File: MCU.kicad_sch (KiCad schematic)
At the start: 13 parts, among them U1 BMD-350-A-R, Y1 32.768kHz

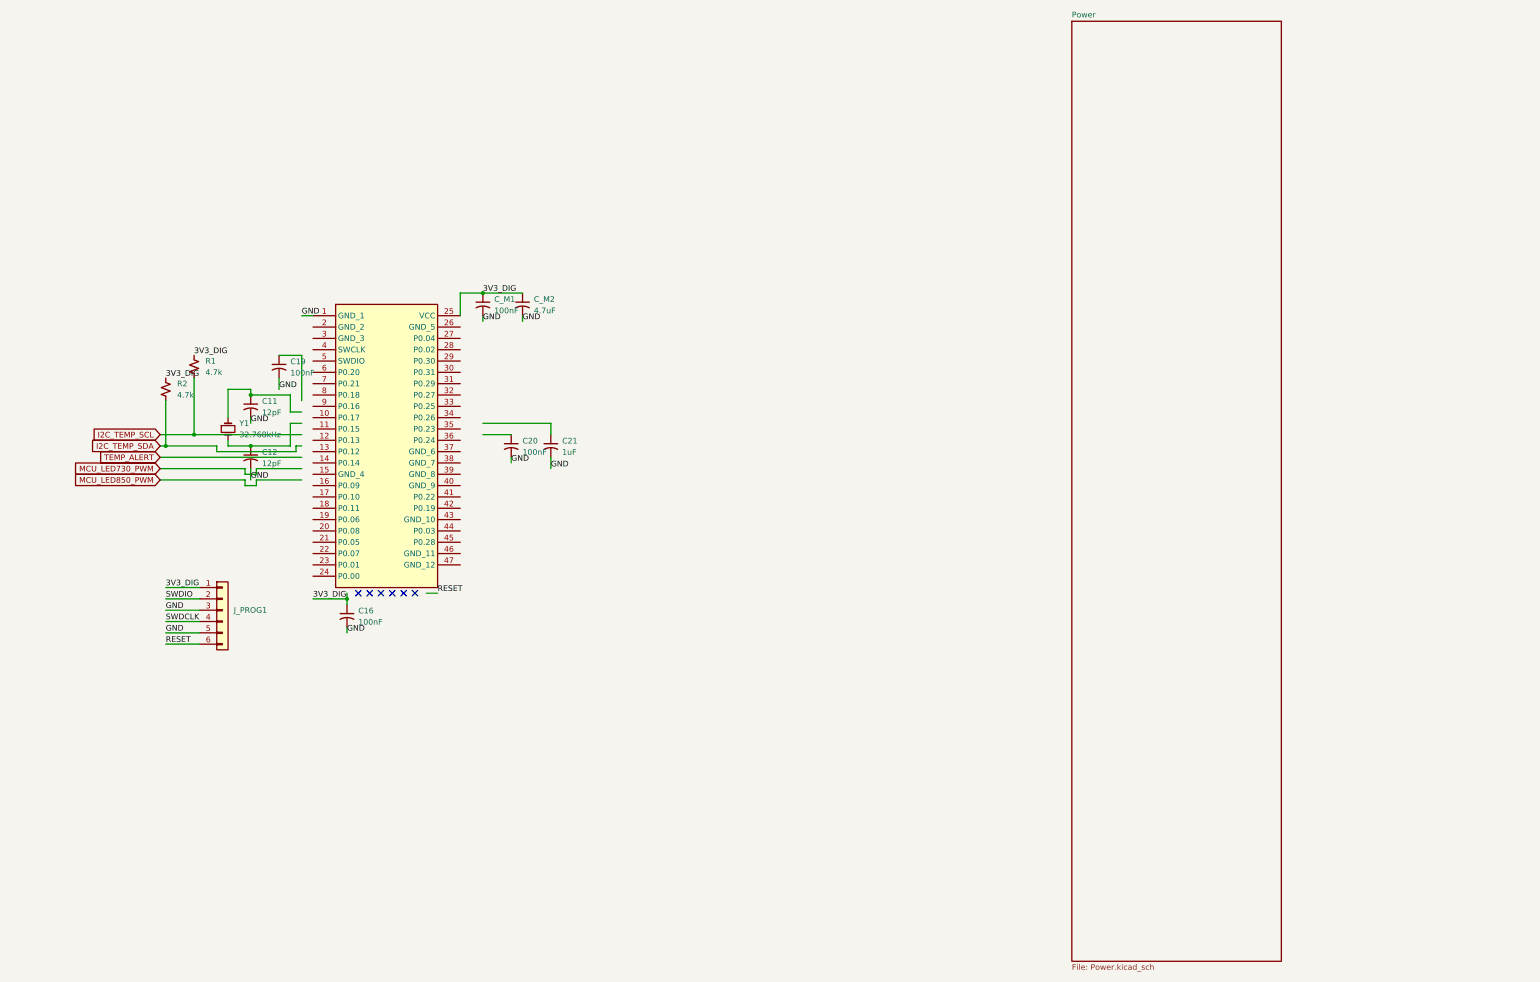
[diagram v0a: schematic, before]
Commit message: power
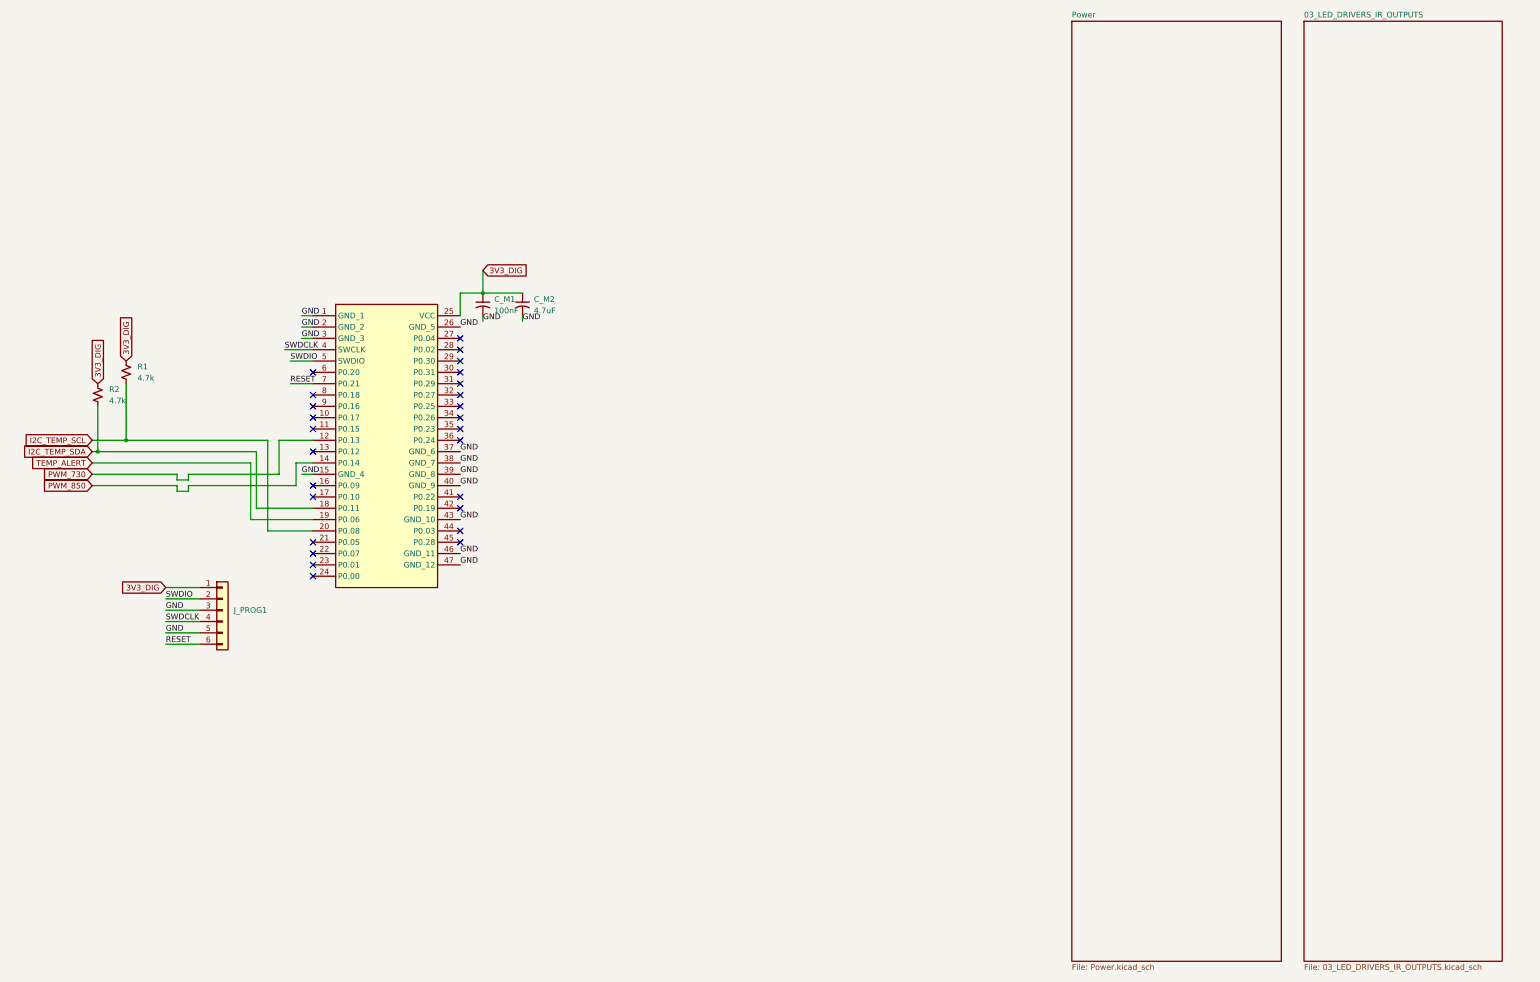
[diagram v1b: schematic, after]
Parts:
- removed C11, C12: 12pF, symbol Device:C_Small_US
- removed C16, C19, C20: 100nF, symbol Device:C_Small_US
- removed C21: 1uF, symbol Device:C_Small_US
- removed Y1: 32.768kHz, symbol Device:Crystal_Small
- U1: footprint BMD-350 -> BMD-350-A-R:BMD-350
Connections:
- net GND: now also U1.15 (GND_4), U1.2 (GND_2), U1.26 (GND_5), U1.3 (GND_3), U1.37 (GND_6), U1.38 (GND_7), U1.39 (GND_8), U1.40 (GND_9), U1.43 (GND_10), U1.46 (GND_11), U1.47 (GND_12)
- net I2C_TEMP_SCL: now also U1.20 (P0.08)
- net I2C_TEMP_SDA: now also U1.18 (P0.11)
- net RESET: now also U1.7 (P0.21)
- net SWDCLK: now also U1.4 (SWCLK)
- net SWDIO: now also U1.5 (SWDIO)
- net TEMP_ALERT: now also U1.19 (P0.06)
- net PWM_730: now reaches U1.12 (P0.13)
- net PWM_850: now reaches U1.14 (P0.14)
- no-connect marks 6 -> 26
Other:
- added sheet 03_LED_DRIVERS_IR_OUTPUTS (03_LED_DRIVERS_IR_OUTPUTS.kicad_sch)
- moved on the sheet: R1, R2
